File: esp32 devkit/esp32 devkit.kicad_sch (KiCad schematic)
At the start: 36 parts, among them Q1 SS8050, Q2 SS8050, SW1 SW_Push, SW2 SW_Push, U1 AMS1117-3.3, U2 ESP32-WROOM-32E(4MB), U3 CP2102N-A02-GQFN28

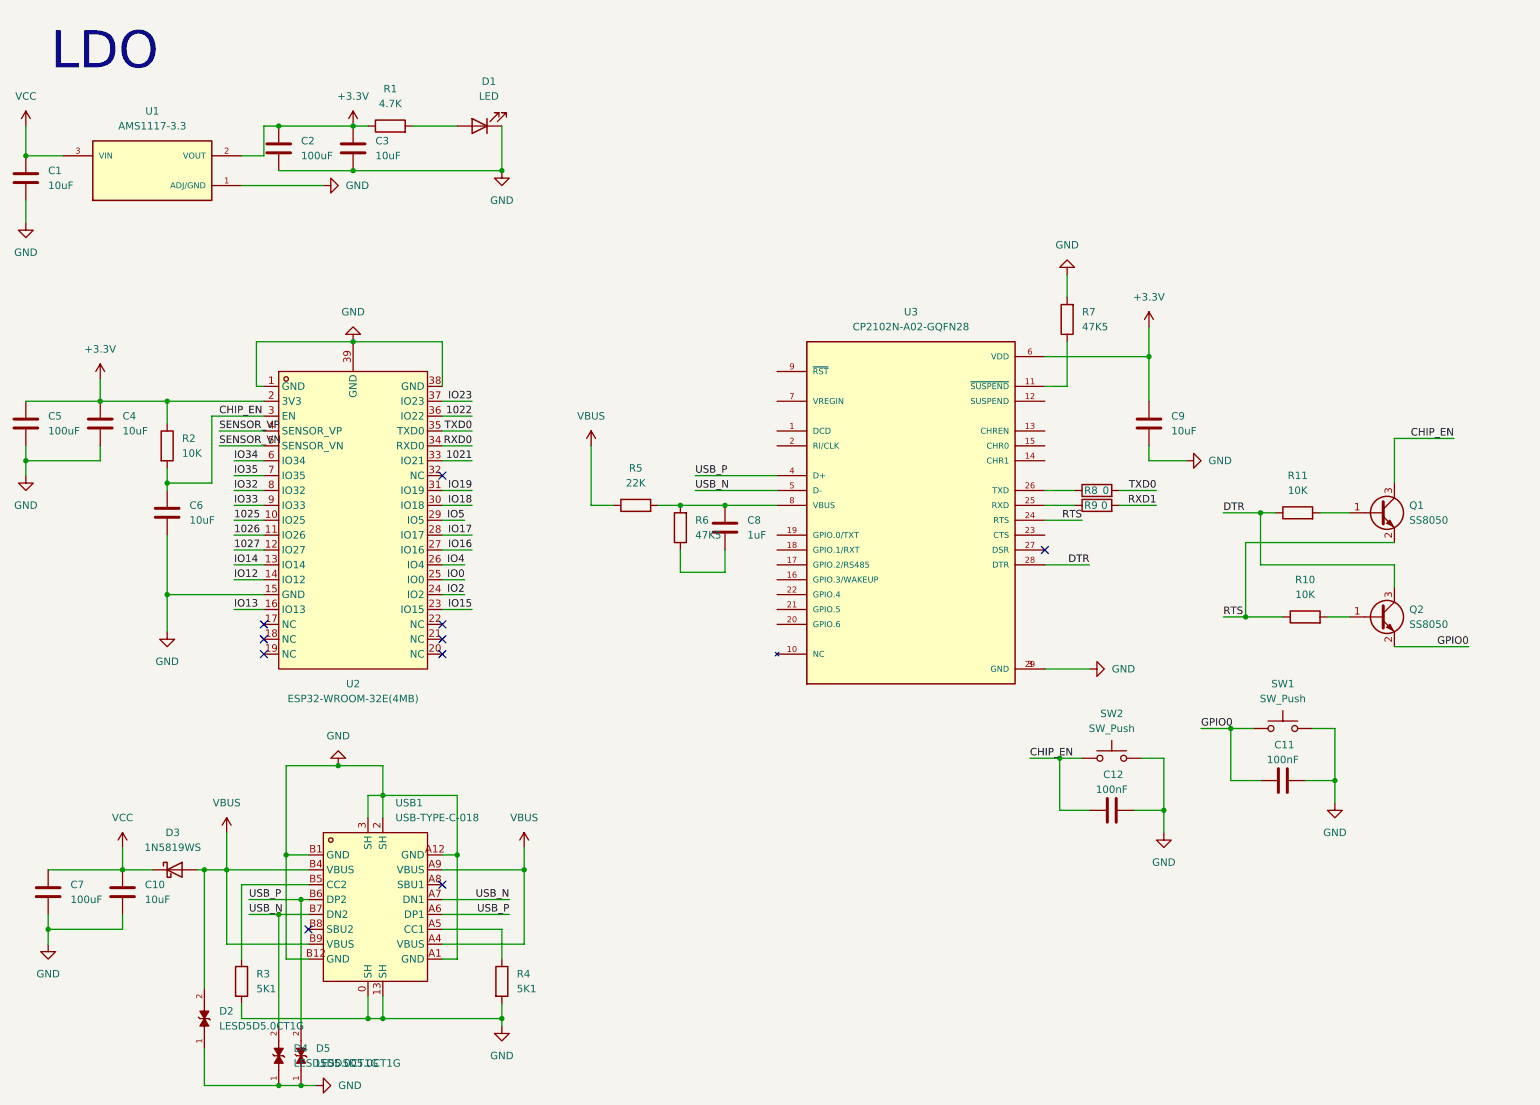
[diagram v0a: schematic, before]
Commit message: :green_heart: completing the connectors
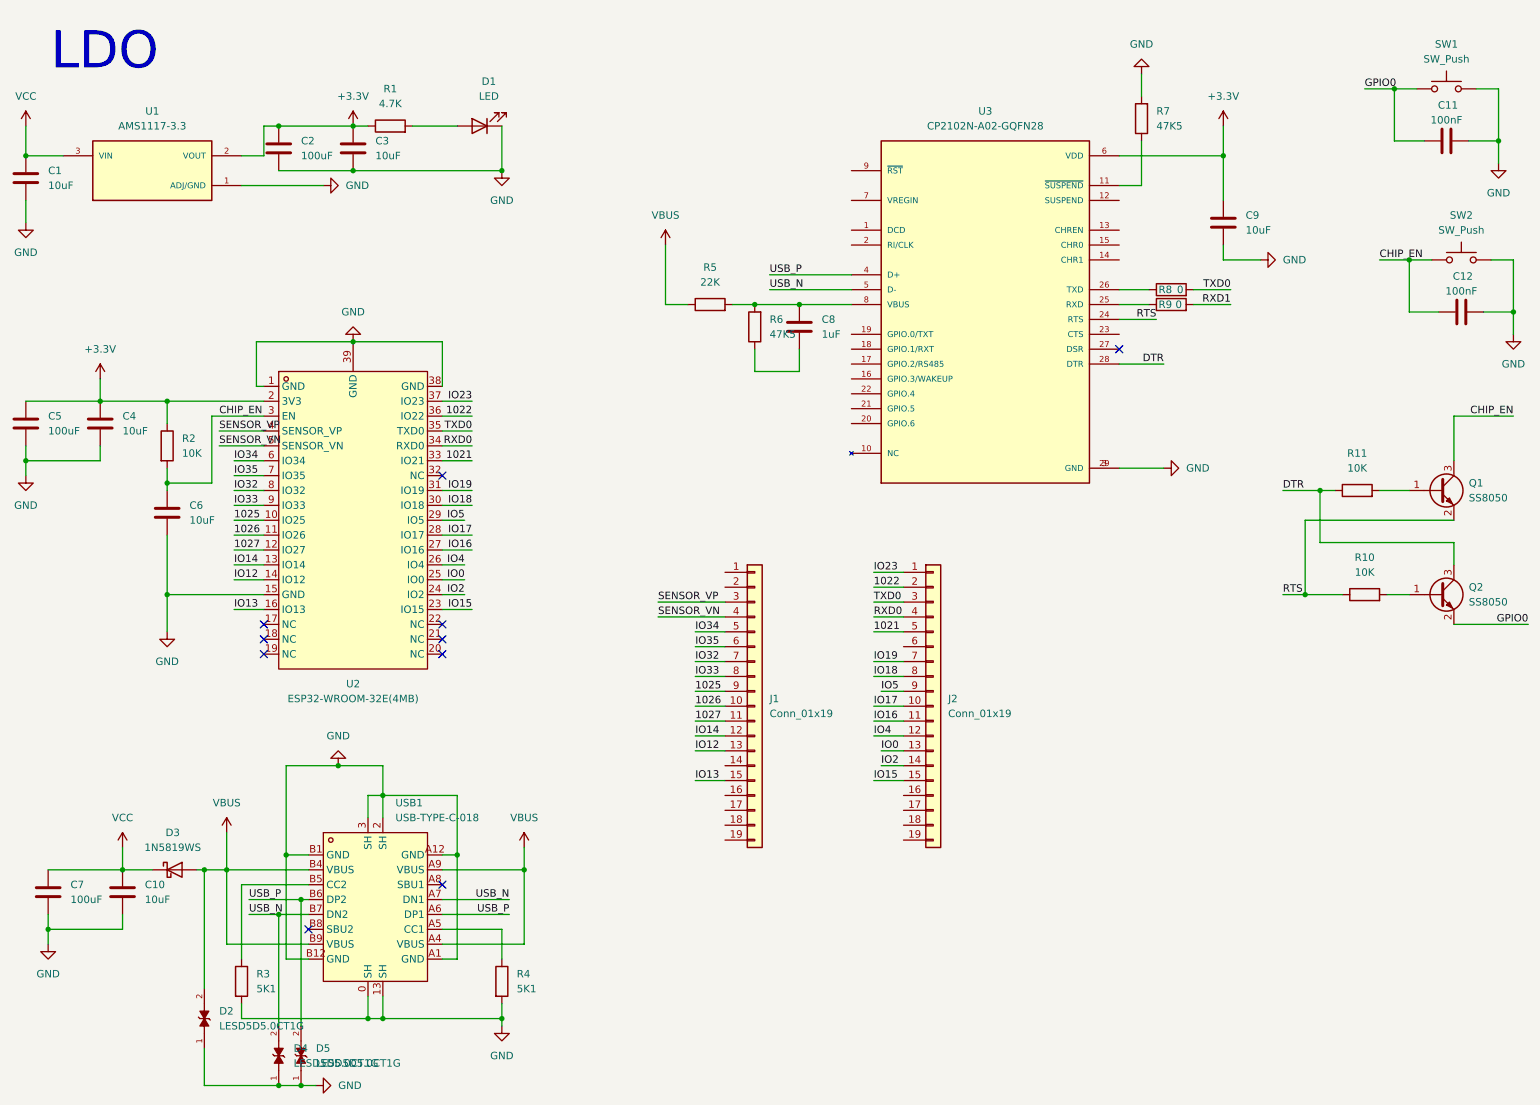
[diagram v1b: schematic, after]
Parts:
- added J1, J2: Conn_01x19, symbol Connector_Generic:Conn_01x19
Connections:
- net 1021: now also J2.5 (Pin_5)
- net 1022: now also J2.2 (Pin_2)
- net 1025: now also J1.9 (Pin_9)
- net 1026: now also J1.10 (Pin_10)
- net 1027: now also J1.11 (Pin_11)
- net IO0: now also J2.13 (Pin_13)
- net IO12: now also J1.13 (Pin_13)
- net IO13: now also J1.15 (Pin_15)
- net IO14: now also J1.12 (Pin_12)
- net IO15: now also J2.15 (Pin_15)
- net IO16: now also J2.11 (Pin_11)
- net IO17: now also J2.10 (Pin_10)
- net IO18: now also J2.8 (Pin_8)
- net IO19: now also J2.7 (Pin_7)
- net IO2: now also J2.14 (Pin_14)
- net IO23: now also J2.1 (Pin_1)
- net IO32: now also J1.7 (Pin_7)
- net IO33: now also J1.8 (Pin_8)
- net IO34: now also J1.5 (Pin_5)
- net IO35: now also J1.6 (Pin_6)
- net IO4: now also J2.12 (Pin_12)
- net IO5: now also J2.9 (Pin_9)
- net RXD0: now also J2.4 (Pin_4)
- net SENSOR_VN: now also J1.4 (Pin_4)
- net SENSOR_VP: now also J1.3 (Pin_3)
- net TXD0: now also J2.3 (Pin_3)
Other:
- moved on the sheet: C11, C12, C8, C9, Q1, Q2, R10, R11, R5, R6, R7, R8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
